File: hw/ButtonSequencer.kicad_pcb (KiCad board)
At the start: 2 copper layers, 76.2 x 99.1 mm, 65 parts, among them J1 clock_in, J2 gate_out_1, J3 gate_out_2, J4 gate_out_3, J5 gate_out_4, J6 power_bus, J7 Conn_02x09_Odd_Even, J8 Conn_02x09_Odd_Even, Q1 2SC1815, SW1 Rotary_Encoder, SW2 enter, SW3 func2, SW4 function, SW5 SW_Push, U1 TL074, U2 ProMicro, U3 74HC595

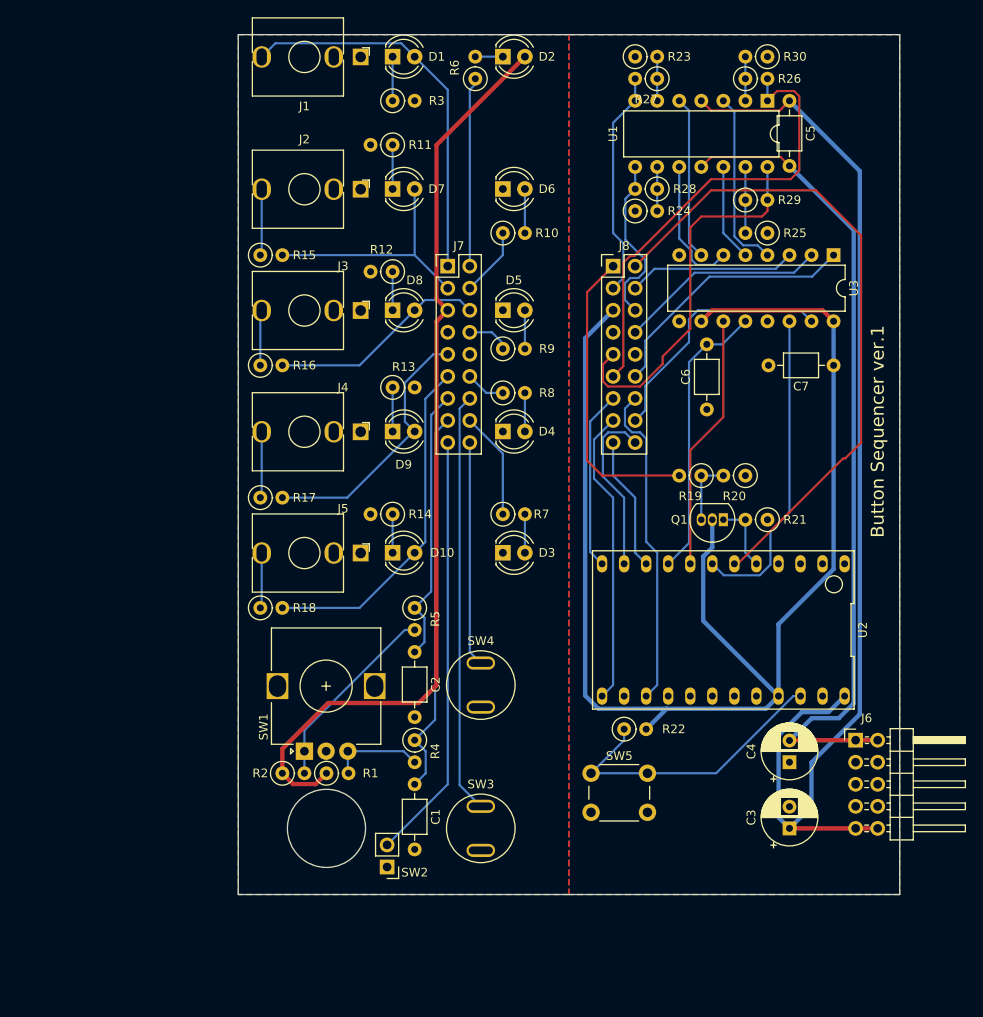
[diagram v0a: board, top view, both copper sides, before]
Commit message: minor mods
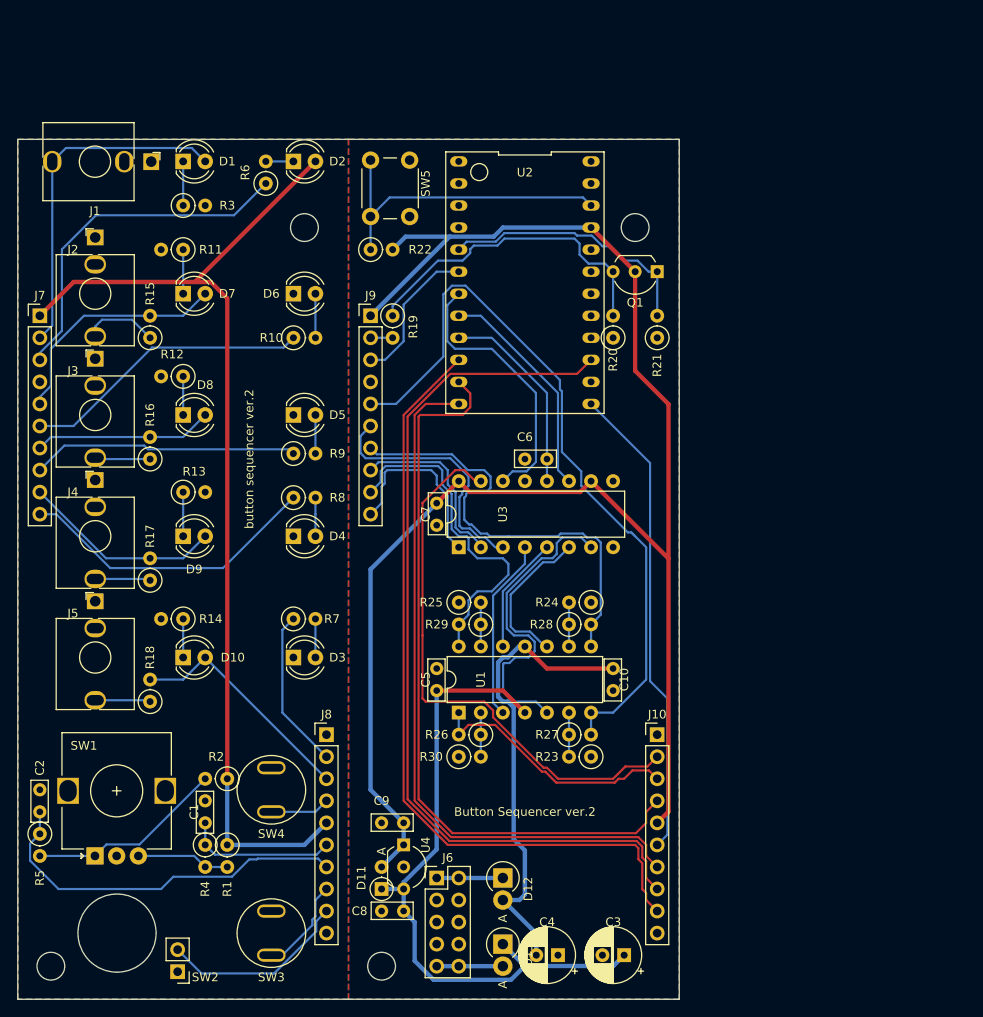
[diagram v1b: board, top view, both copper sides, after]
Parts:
- added C10: 0.1u, Attenuverter:C_Axial_L4.8mm_D2.0mm_P2.54mm_Horizontal, F.Cu at (132.1, 126.4)
- added C8: 0.1u, Attenuverter:C_Axial_L4.8mm_D2.0mm_P2.54mm_Horizontal, F.Cu at (105.4, 151.8)
- added C9: 0.1u, Attenuverter:C_Axial_L4.8mm_D2.0mm_P2.54mm_Horizontal, F.Cu at (105.4, 141.6)
- added D11: 1N4148, Diode_THT:D_DO-35_SOD27_P2.54mm_Vertical_AnodeUp, F.Cu at (105.4, 149.2)
- added D12: D_Schottky, Diode_THT:D_DO-15_P2.54mm_Vertical_AnodeUp, F.Cu at (119.4, 148.0)
- added D13: D_Schottky, Diode_THT:D_DO-15_P2.54mm_Vertical_AnodeUp, F.Cu at (119.4, 155.6)
- added J10: bus_R, Connector_PinHeader_2.54mm:PinHeader_1x10_P2.54mm_Vertical, F.Cu at (137.2, 131.4)
- added J9: bus_L, Connector_PinHeader_2.54mm:PinHeader_1x10_P2.54mm_Vertical, F.Cu at (104.1, 83.2)
- added REF**: MountingHole_3.2mm_M3, MountingHole:MountingHole_3.2mm_M3, F.Cu at (67.3, 158.1)
- added REF**: MountingHole_3.2mm_M3, MountingHole:MountingHole_3.2mm_M3, F.Cu at (96.5, 73.0)
- added REF**: MountingHole_3.2mm_M3, MountingHole:MountingHole_3.2mm_M3, F.Cu at (134.6, 73.0)
- added REF**: MountingHole_3.2mm_M3, MountingHole:MountingHole_3.2mm_M3, F.Cu at (105.4, 158.1)
- added U4: L78L05_TO92, Package_TO_SOT_THT:TO-92_Inline_Wide, F.Cu at (108.0, 144.1)
- C1, C2, C5, C6, C7: footprint Capacitor_THT:C_Axial_L3.8mm_D2.6mm_P7.50mm_Horizontal -> Attenuverter:C_Axial_L4.8mm_D2.0mm_P2.54mm_Horizontal
- J6: footprint Connector_PinHeader_2.54mm:PinHeader_2x05_P2.54mm_Horizontal -> Connector_PinHeader_2.54mm:PinHeader_2x05_P2.54mm_Vertical
- J7: value Conn_02x09_Odd_Even -> bus_L; footprint Connector_PinHeader_2.54mm:PinHeader_2x09_P2.54mm_Vertical -> Connector_PinHeader_2.54mm:PinHeader_1x10_P2.54mm_Vertical
- J8: value Conn_02x09_Odd_Even -> bus_R; footprint Connector_PinHeader_2.54mm:PinHeader_2x09_P2.54mm_Vertical -> Connector_PinHeader_2.54mm:PinHeader_1x10_P2.54mm_Vertical
- Q1: footprint Package_TO_SOT_THT:TO-92_Inline -> Package_TO_SOT_THT:TO-92_Inline_Wide
- moved R26 88.1 mm to (114.3, 134.0), turned to 0 degrees
- moved R30 81.5 mm to (116.8, 131.4), turned to 180 degrees
- moved R23 80.8 mm to (129.5, 134.0), turned to 180 degrees
- moved C5 79.2 mm to (111.8, 126.4), turned to 90 degrees
- moved U1 78.9 mm to (114.3, 128.9), turned to 90 degrees
- moved R27 76.2 mm to (127.0, 131.4), turned to 0 degrees
- moved SW5 69.0 mm to (104.1, 71.8), turned to 90 degrees
- moved J8 63.3 mm to (99.1, 131.4)
- moved R22 62.5 mm to (104.1, 75.6)
- moved R29 57.6 mm to (116.8, 118.7), turned to 180 degrees
- moved R25 55.4 mm to (114.3, 116.2), turned to 0 degrees
- moved U3 54.7 mm to (114.3, 109.9), turned to 90 degrees
- moved R28 51.2 mm to (127.0, 118.7), turned to 0 degrees
- moved J6 50.8 mm to (111.8, 148.0)
- moved R5 50.4 mm to (66.0, 142.9)
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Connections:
- C5 pad 2: -12V -> GND
- J6 pad 1: -12V -> Net-(D12-Pad1)
- J6 pad 10: +12V -> Net-(D13-Pad2)
- J6 pad 2: -12V -> Net-(D12-Pad1)
- J6 pad 9: +12V -> Net-(D13-Pad2)
- J7 pad 1: /Sheet62419879/clock_in -> +5V
- J7 pad 10: GND -> /Sheet62419879/select_3
- J7 pad 2: /Sheet62419879/seq_start -> /Sheet62419879/clock_in
- J7 pad 3: /Sheet62419879/gate_1 -> /Sheet62419879/seq_start
- J7 pad 4: /Sheet62419879/select_1 -> GND
- J7 pad 5: +5V -> /Sheet62419879/gate_1
- J7 pad 6: /Sheet62419879/gate_2 -> /Sheet62419879/select_1
- J7 pad 7: GND -> /Sheet62419879/gate_2
- J8 pad 1: /Sheet62451AD7/clock_in -> GND
- J8 pad 2: /Sheet62451AD7/seq_start -> /Sheet62419879/select_4
- J8 pad 3: /Sheet62451AD7/gate_1 -> /Sheet62419879/gate_4
- J8 pad 4: /Sheet62451AD7/select_1 -> /Sheet62419879/sw_func_1
- J8 pad 6: /Sheet62451AD7/gate_2 -> /Sheet62419879/re_2
- J8 pad 7: GND -> /Sheet62419879/re_1
- J8 pad 8: /Sheet62451AD7/select_2 -> /Sheet62419879/sw_func_2
- J8 pad 9: /Sheet62451AD7/gate_3 -> /Sheet62419879/sw_enter
- U2 pad 24: +12V -> Net-(U2-Pad24)
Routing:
- net /Sheet62451AD7/sw_enter: track 15.5 -> 90.9 mm
- net /Sheet62451AD7/sw_func_1: track 20.0 -> 85.5 mm
- net /Sheet62451AD7/sw_func_2: track 37.4 -> 102.8 mm
- net /Sheet62451AD7/re_1: track 20.7 -> 81.9 mm
- net /Sheet62451AD7/gate_1: track 26.2 -> 85.9 mm
- net /Sheet62451AD7/seq_start: track 76.1 -> 16.8 mm
- net +12V: track 132.5 -> 76.8 mm
- net +5V: track 266.4 -> 308.9 mm
- net -12V: track 95.4 -> 54.2 mm
- net /Sheet62419879/sw_func_2: track 48.5 -> 11.0 mm
- net /Sheet62451AD7/select_4: track 29.3 -> 63.7 mm
- net /Sheet62451AD7/clock_in: track 35.0 -> 2.54 mm
- net /Sheet62451AD7/gate_2: track 19.9 -> 52.2 mm
- net /Sheet62419879/select_3: track 4.60 -> 35.1 mm
- net Net-(Q1-Pad3): track 7.62 -> 37.4 mm
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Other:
- board text added: "Button Sequencer ver.2"
- board text added: "button sequencer ver.2"
- board text removed: "Button Sequencer ver.1"
